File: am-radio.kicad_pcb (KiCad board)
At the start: 2 copper layers, 180 x 62 mm, 51 parts, among them J1 SPEAKER 8R, Q1 2N3904, Q2 2N3904, Q3 2N3904, Q4 2N3904, Q5 2N3904, Q6 2N3904, SW1 POWER, T1 42IF101 (yellow), T2 42IF102 (white), T3 42IF103 (black), T4 42TU013, T5 42TU200

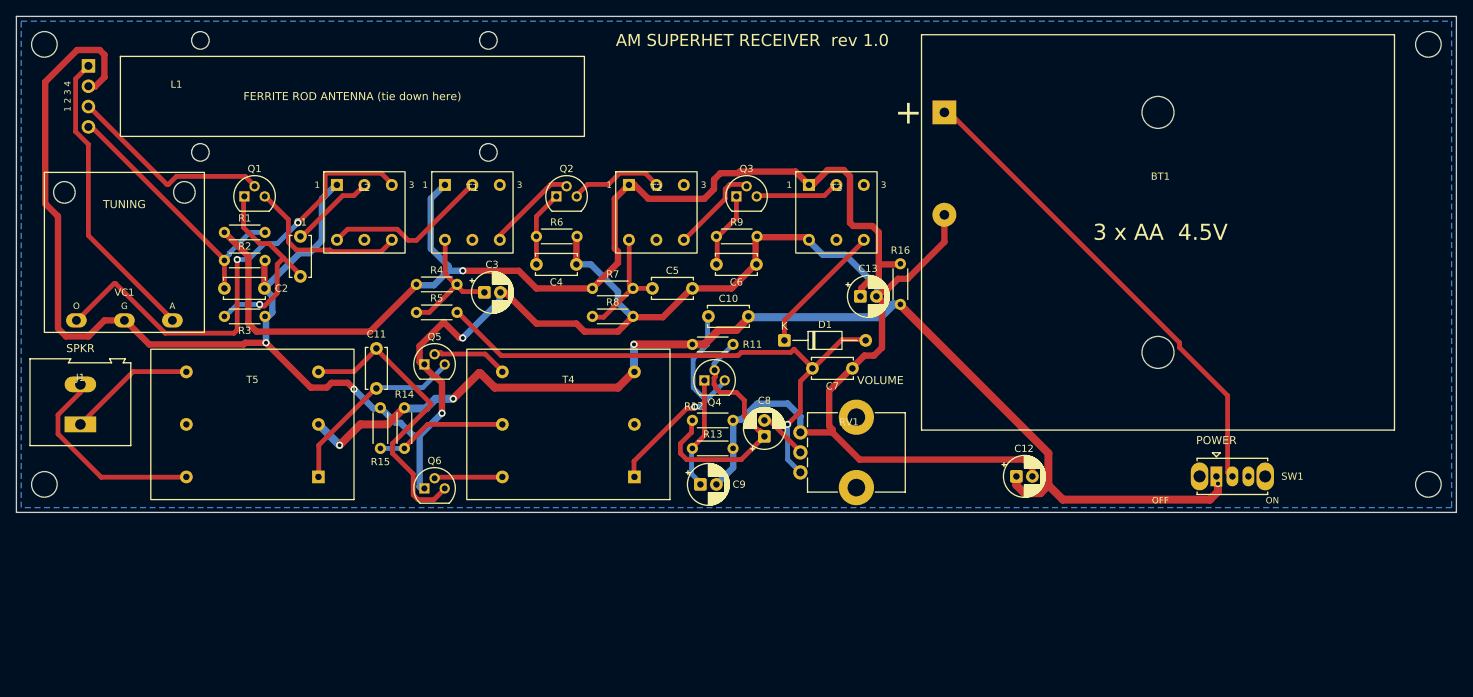
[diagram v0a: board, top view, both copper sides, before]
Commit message: checkpoint
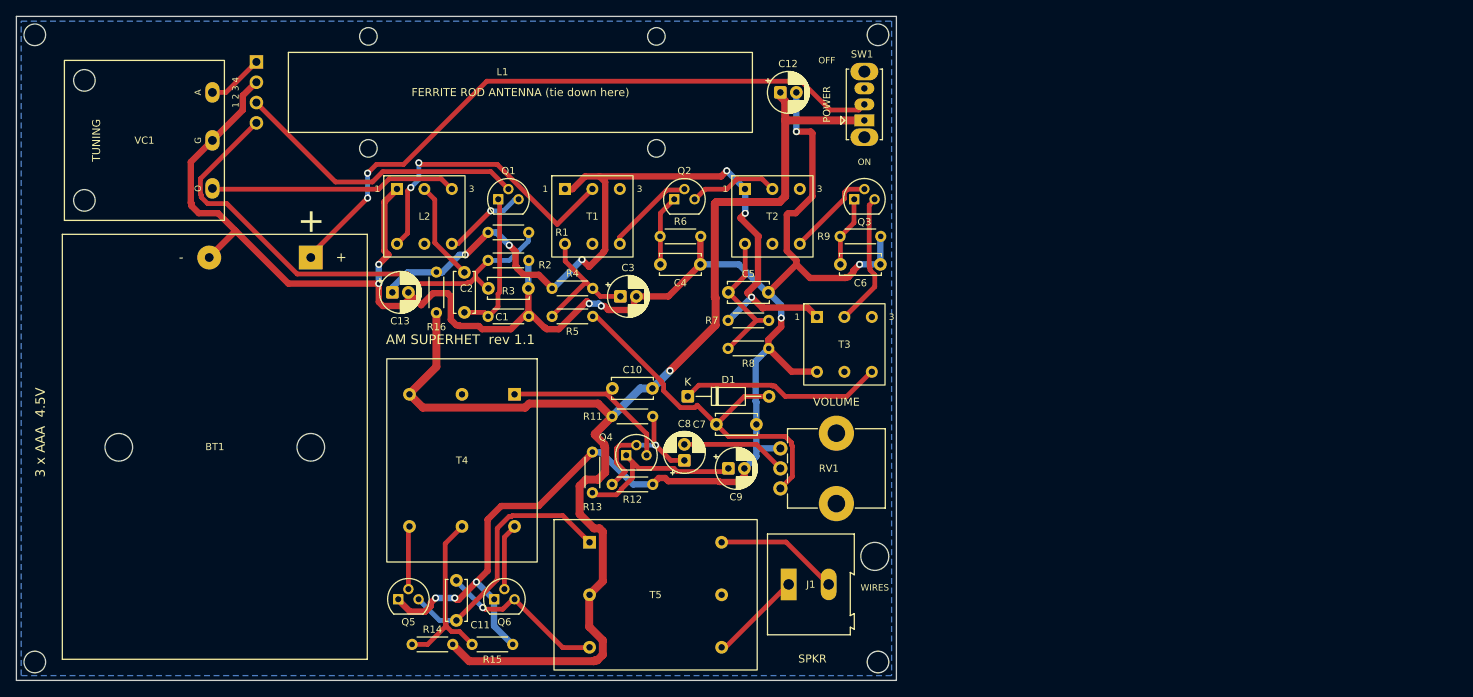
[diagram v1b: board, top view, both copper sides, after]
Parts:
- BT1: value 3xAA 4.5V -> 3xAAA 4.5V; footprint BatteryHolder_TruPower_BH-331P_3xAA -> Battery:BatteryHolder_Keystone_2479_3xAAA
- C1, C10, C11, C2, C4, C5, C6, C7: footprint C_Disc_D5.0mm_W2.5mm_P5.00mm -> Capacitor_THT:C_Disc_D5.0mm_W2.5mm_P5.00mm
- C12, C13, C3, C8, C9: footprint CP_Radial_D5.0mm_P2.00mm -> Capacitor_THT:CP_Radial_D5.0mm_P2.00mm
- D1: footprint D_DO-35_SOD27_P10.16mm_Horizontal -> Diode_THT:D_DO-35_SOD27_P10.16mm_Horizontal
- H1, H2, H3, H4: value M3 -> M2.5; footprint MountingHole_3.2mm_M3 -> MountingHole:MountingHole_2.7mm_M2.5
- J1: footprint TerminalBlock_Altech_AK300-2_P5.00mm -> TerminalBlock:TerminalBlock_Altech_AK300-2_P5.00mm
- L1: footprint Ferrite_Rod_Antenna_Coil -> audio:Ferrite_Rod_Antenna_Coil
- L2, T1, T2, T3: footprint Xicon_42IF10x -> audio:Xicon_42IF10x
- Q1, Q2, Q3, Q4, Q5, Q6: footprint TO-92 -> Package_TO_SOT_THT:TO-92
- R1, R11, R12, R13, R14, R15, R16, R2, R3, R4, R5, R6, R7, R8, R9: footprint R_Axial_DIN0204_L3.6mm_D1.6mm_P5.08mm_Horizontal -> Resistor_THT:R_Axial_DIN0204_L3.6mm_D1.6mm_P5.08mm_Horizontal
- RV1: footprint Potentiometer_Bourns_PTV09A-1_Single_Vertical -> Potentiometer_THT:Potentiometer_Bourns_PTV09A-1_Single_Vertical
- SW1: footprint SW_Slide_SPDT_Straight_CK_OS102011MS2Q -> Button_Switch_THT:SW_Slide_SPDT_Straight_CK_OS102011MS2Q
- T4, T5: footprint Xicon_42TU200-RC -> audio:Xicon_42TU200-RC
- VC1: footprint Polyvaricon_CBM-223P_Wired -> audio:Polyvaricon_CBM-223P_Wired
- moved J1 90.8 mm to (116.5, 91.0), turned to 0 degrees
- moved BT1 81.3 mm to (56.8, 50.1), turned to -90 degrees
- moved H4 72.3 mm to (127.7, 100.7)
- moved H2 68.8 mm to (127.7, 22.3)
- moved SW1 62.6 mm to (126.0, 33.0), turned to 90 degrees
- moved C13 58.5 mm to (67.0, 54.5)
- moved R16 58.0 mm to (72.5, 57.0)
- moved C12 56.3 mm to (115.5, 29.5)
- moved T5 54.7 mm to (99.9, 92.3), turned to 0 degrees
- moved C2 33.0 mm to (79.0, 54.0)
- moved R1 33.0 mm to (79.0, 47.0)
- moved R2 33.0 mm to (79.0, 50.5)
- moved R3 33.0 mm to (79.0, 57.5)
- moved Q1 31.7 mm to (80.2, 42.9)
- moved C11 30.7 mm to (75.0, 95.5)
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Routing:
- net V_RF: track 141.9 -> 99.7 mm, vias 1 -> 6
- net GND: track 326.4 -> 290.3 mm, vias 4 -> 10
- net Net-(VC1-A): track 37.5 -> 7.07 mm
- net Net-(C2-Pad1): track 34.0 -> 63.4 mm
- net Net-(VC1-O): track 59.4 -> 31.0 mm, vias 2 -> 0
- net /DET: track 71.2 -> 46.6 mm, vias 1 -> 0
- net Net-(BT1-+): track 60.9 -> 82.1 mm, vias 0 -> 2
- net Net-(L2-Pad6): track 21.1 -> 37.9 mm, vias 0 -> 2
- net Net-(Q6-C): track 37.3 -> 21.3 mm, vias 0 -> 1
- net +BATT: track 144.8 -> 160.2 mm, vias 4 -> 1
- net Net-(Q4-B): track 33.5 -> 18.8 mm, vias 0 -> 1
- net Net-(Q1-B): track 25.8 -> 37.1 mm
- net Net-(Q1-C): track 21.1 -> 10.7 mm, vias 0 -> 1
- net Net-(J1-Pin_2): track 25.6 -> 15.6 mm
- net Net-(Q5-C): track 23.9 -> 33.0 mm
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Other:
- board size 180 x 62 mm -> 110 x 83 mm
- board text added: "+"
- board text added: "-"
- board text added: "3 x AAA 4.5V"
- board text added: "AM SUPERHET rev 1.1"
- board text added: "WIRES"
- board text added: "am-radio rev 1.1 2026-09"
- board text removed: "3 x AA 4.5V"
- board text removed: "AM SUPERHET RECEIVER rev 1.0"
- board text removed: "am-radio rev 1.0 2026-09"
